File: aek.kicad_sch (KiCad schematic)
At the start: 239 parts, among them J1 Conn_01x04_MountingPin, SW1 SW_Push, U1 ATmega32U4-AU, Y1 16MHz

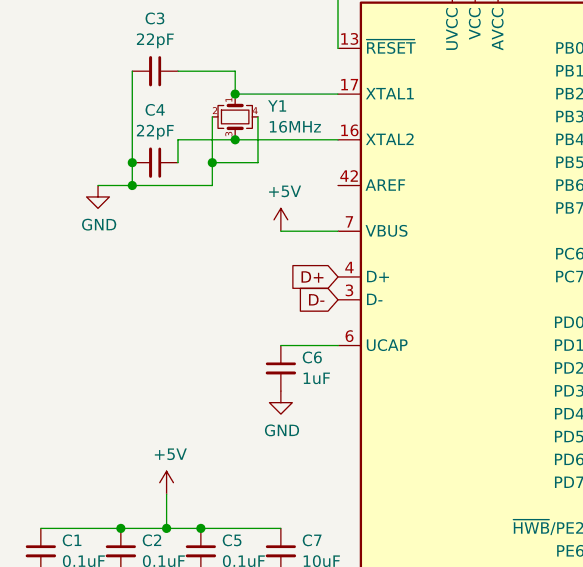
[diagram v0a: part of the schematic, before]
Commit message: updates
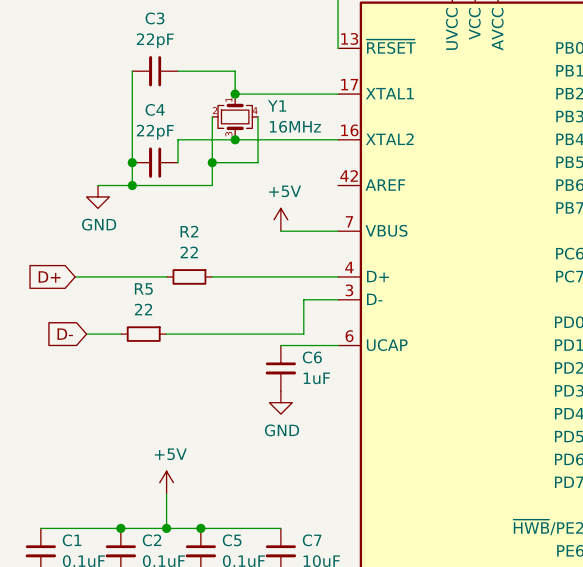
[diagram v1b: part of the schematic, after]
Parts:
- added R2, R5: 22, Resistor_SMD:R_0805_2012Metric, symbol Device:R_Small
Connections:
- net D+: now also R2.2; no longer U1.4 (D+)
- net D-: now also R5.2; no longer U1.3 (D-)
- new net: R5.1, U1.3 (D-)
- new net: R2.1, U1.4 (D+)
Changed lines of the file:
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@@
     (stroke (width 0) (type solid) (color 0 0 0 0))
   )
+  (wire (pts (xy 27.94 85.09) (xy 38.1 85.09))
+    (stroke (width 0) (type solid) (color 0 0 0 0))
+  )
+  (wire (pts (xy 29.21 91.44) (xy 33.02 91.44))
+    (stroke (width 0) (type solid) (color 0 0 0 0))
+  )
   (wire (pts (xy 29.21 233.68) (xy 29.21 241.3))
     (stroke (width 0) (type solid) (color 0 0 0 0))
@@
     (stroke (width 0) (type solid) (color 0 0 0 0))
   )
+  (wire (pts (xy 38.1 91.44) (xy 53.34 91.44))
+    (stroke (width 0) (type solid) (color 0 0 0 0))
+  )
   (wire (pts (xy 38.1 113.03) (xy 38.1 109.22))
     (stroke (width 0) (type solid) (color 0 0 0 0))
@@
     (stroke (width 0) (type solid) (color 0 0 0 0))
   )
+  (wire (pts (xy 43.18 85.09) (xy 57.15 85.09))
+    (stroke (width 0) (type solid) (color 0 0 0 0))
+  )
   (wire (pts (xy 45.72 62.23) (xy 45.72 64.77))
     (stroke (width 0) (type solid) (color 0 0 0 0))
@@
     (stroke (width 0) (type solid) (color 0 0 0 0))
   )
+  (wire (pts (xy 53.34 87.63) (xy 57.15 87.63))
+    (stroke (width 0) (type solid) (color 0 0 0 0))
+  )
+  (wire (pts (xy 53.34 91.44) (xy 53.34 87.63))
+    (stroke (width 0) (type solid) (color 0 0 0 0))
+  )
   (wire (pts (xy 54.61 259.08) (xy 54.61 254))
     (stroke (width 0) (type solid) (color 0 0 0 0))
@@
     (stroke (width 0) (type solid) (color 0 0 0 0))
   )
-  (global_label "D-" (shape input) (at 38.1 177.8 180) (fields_autoplaced)
+  (global_label "D+" (shape input) (at 27.94 85.09 180) (fields_autoplaced)
     (effects (font (size 1.27 1.27)) (justify right))
-    (property "Intersheet References" "${INTERSHEET_REFS}" (id 0) (at 0 -39.37 0)
+    (property "Intersheet References" "${INTERSHEET_REFS}" (id 0) (at -21.59 -41.91 0)
       (effects (font (size 1.27 1.27)) hide)
     )
   )
-  (global_label "D+" (shape input) (at 38.1 180.34 180) (fields_autoplaced)
+  (global_label "D-" (shape input) (at 29.21 91.44 180) (fields_autoplaced)
     (effects (font (size 1.27 1.27)) (justify right))
-    (property "Intersheet References" "${INTERSHEET_REFS}" (id 0) (at 0 -39.37 0)
+    (property "Intersheet References" "${INTERSHEET_REFS}" (id 0) (at -20.32 -38.1 0)
       (effects (font (size 1.27 1.27)) hide)
     )
   )
-  (global_label "D+" (shape input) (at 57.15 85.09 180) (fields_autoplaced)
+  (global_label "D-" (shape input) (at 38.1 177.8 180) (fields_autoplaced)
     (effects (font (size 1.27 1.27)) (justify right))
-    (property "Intersheet References" "${INTERSHEET_REFS}" (id 0) (at 7.62 -41.91 0)
+    (property "Intersheet References" "${INTERSHEET_REFS}" (id 0) (at 0 -39.37 0)
       (effects (font (size 1.27 1.27)) hide)
     )
   )
-  (global_label "D-" (shape input) (at 57.15 87.63 180) (fields_autoplaced)
+  (global_label "D+" (shape input) (at 38.1 180.34 180) (fields_autoplaced)
     (effects (font (size 1.27 1.27)) (justify right))
-    (property "Intersheet References" "${INTERSHEET_REFS}" (id 0) (at 7.62 -41.91 0)
+    (property "Intersheet References" "${INTERSHEET_REFS}" (id 0) (at 0 -39.37 0)
       (effects (font (size 1.27 1.27)) hide)
     )
@@
     (pin "1")
   )
+  (symbol (lib_id "Device:R_Small") (at 35.56 91.44 270) (unit 1)
+    (in_bom yes) (on_board yes)
+    (property "Reference" "R5" (id 0) (at 35.56 86.4616 90))
+    (property "Value" "22" (id 1) (at 35.56 88.773 90))
+    (property "Footprint" "Resistor_SMD:R_0805_2012Metric" (id 2) (at 35.56 91.44 0)
+      (effects (font (size 1.27 1.27)) hide)
+    )
+    (property "Datasheet" "~" (id 3) (at 35.56 91.44 0)
+      (effects (font (size 1.27 1.27)) hide)
+    )
+    (pin "1")
+    (pin "2")
+  )
+  (symbol (lib_id "Device:R_Small") (at 40.64 85.09 270) (unit 1)
+    (in_bom yes) (on_board yes)
+    (property "Reference" "R2" (id 0) (at 40.64 80.1116 90))
+    (property "Value" "22" (id 1) (at 40.64 82.423 90))
+    (property "Footprint" "Resistor_SMD:R_0805_2012Metric" (id 2) (at 40.64 85.09 0)
+      (effects (font (size 1.27 1.27)) hide)
+    )
+    (property "Datasheet" "~" (id 3) (at 40.64 85.09 0)
+      (effects (font (size 1.27 1.27)) hide)
+    )
+    (pin "1")
+    (pin "2")
+  )
   (symbol (lib_id "Device:R_Small") (at 57.15 39.37 180) (unit 1)
     (in_bom yes) (on_board yes)
@@
       (reference "R1") (unit 1) (value "330") (footprint "Resistor_SMD:R_0805_2012Metric")
     )
+    (path "/370e7d12-ac1a-44b1-8214-0db731e008f1"
+      (reference "R2") (unit 1) (value "22") (footprint "Resistor_SMD:R_0805_2012Metric")
+    )
     (path "/00000000-0000-0000-0000-000061280f1c"
       (reference "R3") (unit 1) (value "10k") (footprint "Resistor_SMD:R_0805_2012Metric")
@@
       (reference "R4") (unit 1) (value "10k") (footprint "Resistor_SMD:R_0805_2012Metric")
     )
+    (path "/86f546b5-aa43-4d36-9777-f9e527e27aec"
+      (reference "R5") (unit 1) (value "22") (footprint "Resistor_SMD:R_0805_2012Metric")
+    )
     (path "/00000000-0000-0000-0000-00006127121f"
